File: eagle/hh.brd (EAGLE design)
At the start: 169.7 x 51.9 mm, 7 parts

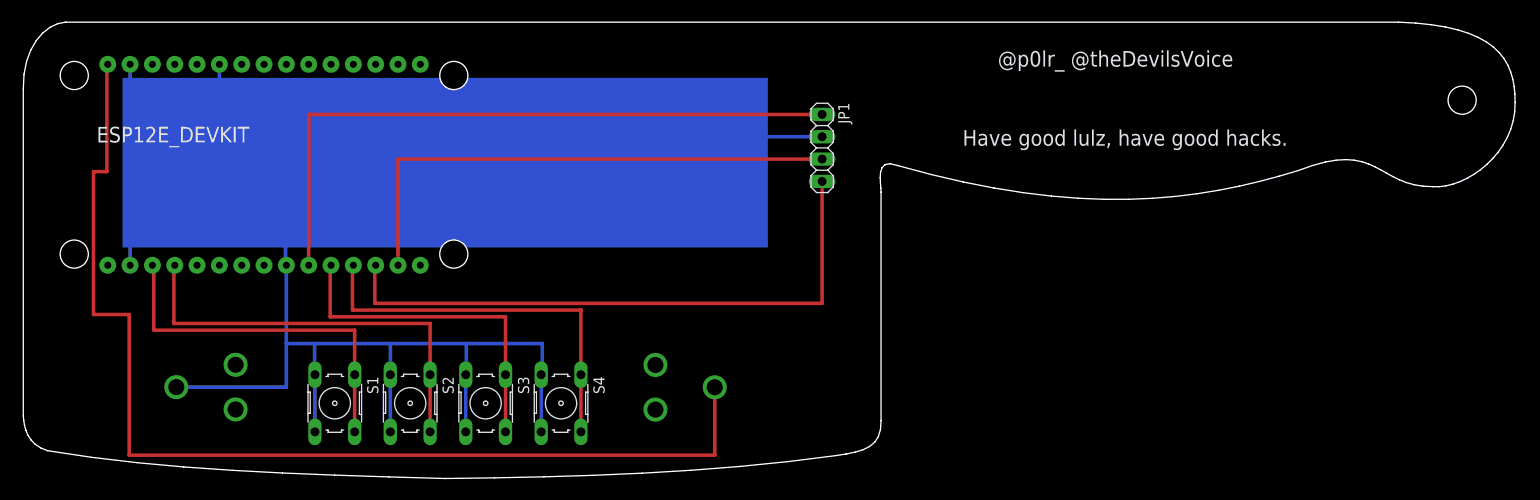
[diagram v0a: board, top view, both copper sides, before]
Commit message: Add files via upload
Latest Update
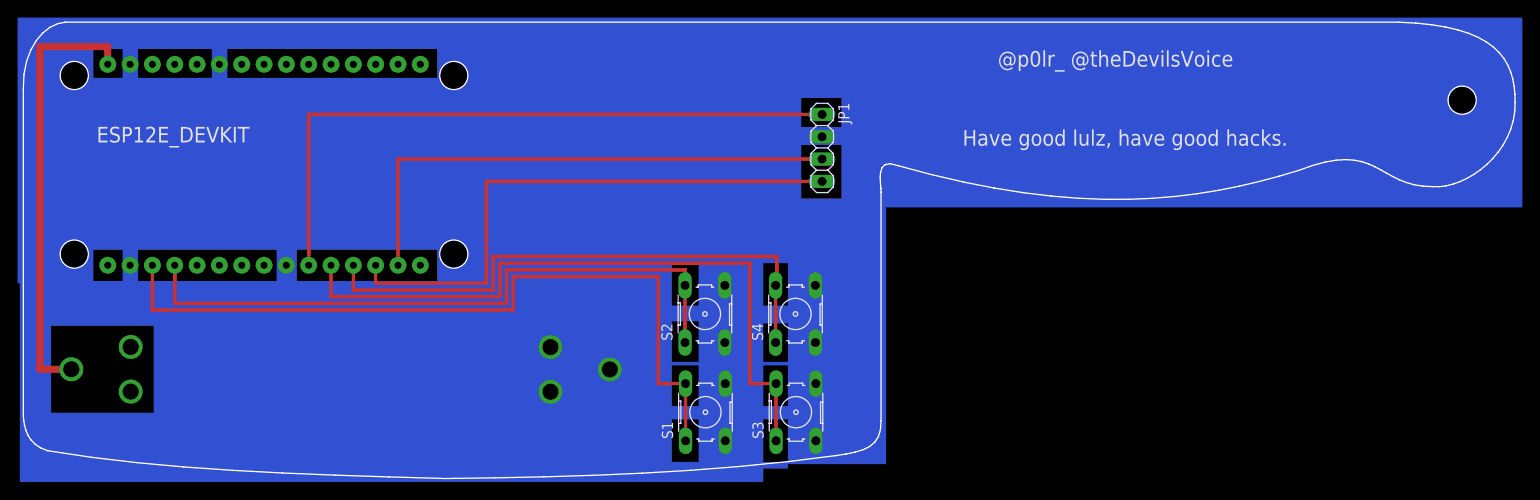
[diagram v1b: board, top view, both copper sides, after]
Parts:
- moved S1 42.2 mm to (77.7, 7.68), turned to 90 degrees
- moved S3 35.3 mm to (88.0, 7.68), turned to 90 degrees
- moved S2 35.0 mm to (77.7, 18.9), turned to 90 degrees
- moved S4 28.5 mm to (88.0, 18.9), turned to 90 degrees
- moved BAT1 12.1 mm to (36.2, 12.6), turned to 180 degrees
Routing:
- net N$4: track 124.5 -> 50.0 mm
- net N$9: track 42.3 -> 88.2 mm
- net N$1: track 220.5 -> 262.4 mm
- net N$7: track 39.3 -> 78.2 mm
- net N$8: track 48.6 -> 74.5 mm
- net N$2: track 45.1 -> 64.7 mm
- net N$6: track 69.2 -> 64.4 mm
